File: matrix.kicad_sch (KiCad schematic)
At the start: 94 parts, among them SW10 K08, SW11 K09, SW12 K0A, SW13 K0B, SW14 K0C, SW15 K10, SW16 K11, SW17 K12, SW18 K13, SW19 K14, SW2 K00, SW20 K15, SW21 K16, SW22 K17, SW23 K18, SW24 K19, SW25 K1A, SW26 K1B, SW27 K20, SW28 K21, SW29 K22, SW3 K01, SW30 K23, SW31 K24, SW32 K25, SW33 K26, SW34 K27, SW35 K28, SW36 K29, SW37 K2A, SW38 K2B, SW39 K30, SW4 K02, SW40 K31, SW41 K32, SW42 K33, SW43 K34, SW44 K36, SW45 K38, SW46 K39, SW47 K3A, SW48 K3B, SW5 K03, SW6 K04, SW7 K05, SW8 K06, SW9 K07

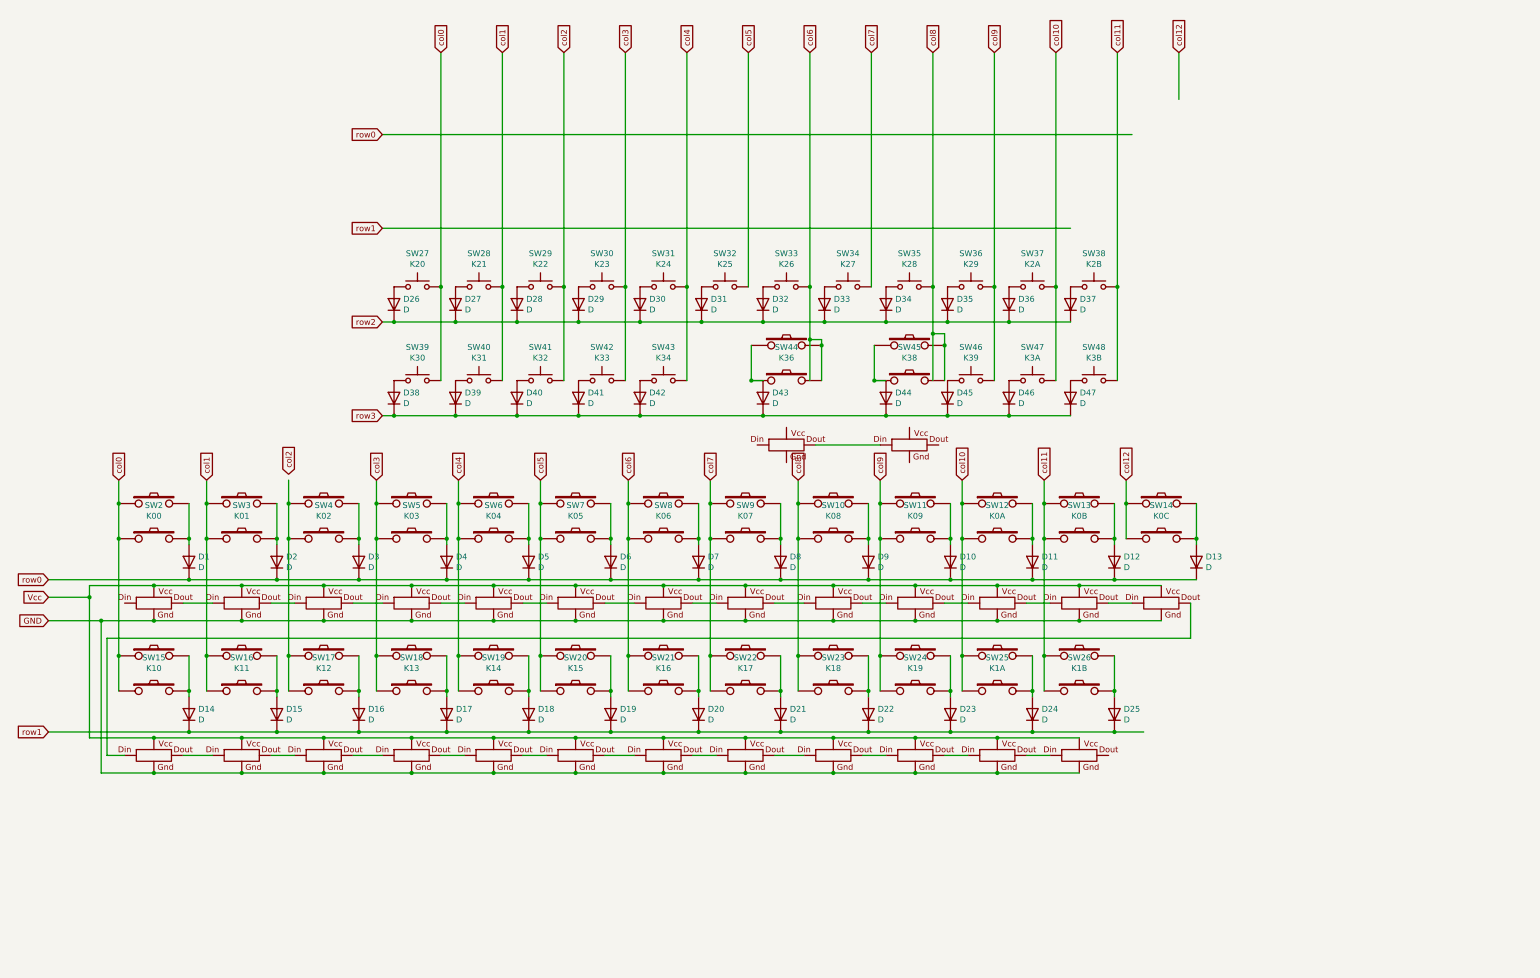
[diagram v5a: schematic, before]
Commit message: routing lol
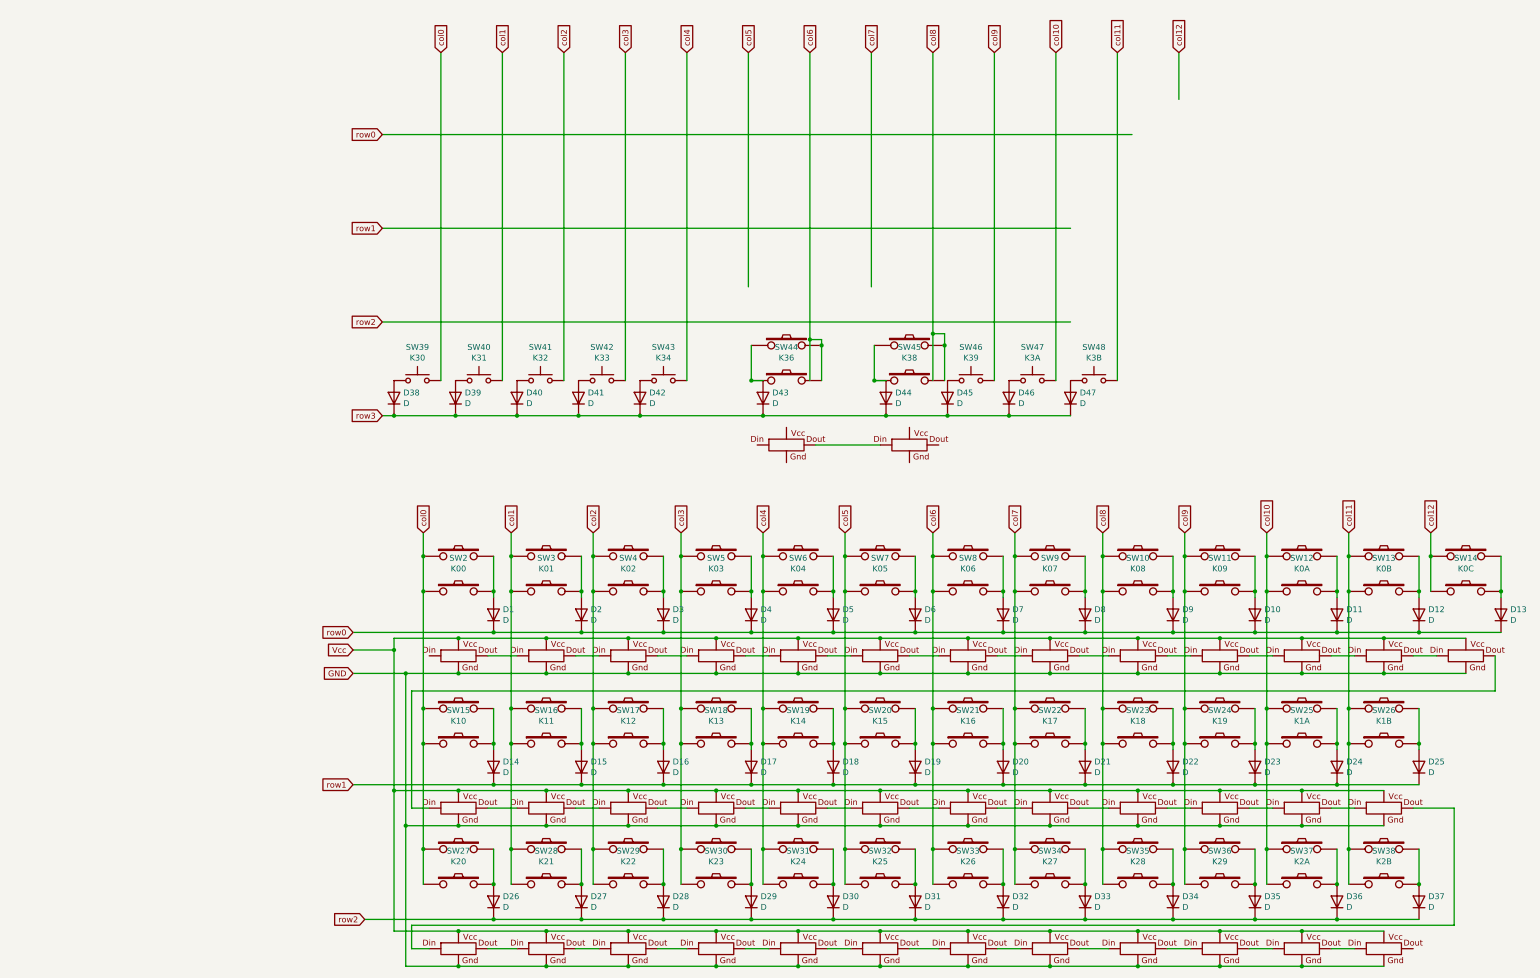
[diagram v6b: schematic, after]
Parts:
- SW27, SW28, SW29, SW30, SW31, SW32, SW33, SW34, SW35, SW36, SW37, SW38: symbol Switch:SW_Push -> switches:SWITCH_PUSH_MXCHOC
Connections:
- net GND: now also SW27.12 (VSS), SW28.12 (VSS), SW29.12 (VSS), SW30.12 (VSS), SW31.12 (VSS), SW32.12 (VSS), SW33.12 (VSS), SW34.12 (VSS), SW35.12 (VSS), SW36.12 (VSS), SW37.12 (VSS), SW38.12 (VSS)
- net Vcc: now also SW27.10 (Vdd), SW28.10 (Vdd), SW29.10 (Vdd), SW30.10 (Vdd), SW31.10 (Vdd), SW32.10 (Vdd), SW33.10 (Vdd), SW34.10 (Vdd), SW35.10 (Vdd), SW36.10 (Vdd), SW37.10 (Vdd), SW38.10 (Vdd)
- net col0: now also SW27.1, SW27.3; no longer SW27.2
- net col1: now also SW28.1, SW28.3; no longer SW28.2
- net col10: now also SW37.1, SW37.3; no longer SW37.2
- net col11: now also SW38.1, SW38.3; no longer SW38.2
- net col2: now also SW17.1, SW17.3, SW29.1, SW29.3, SW4.1, SW4.3; no longer SW29.2
- net col3: now also SW30.1, SW30.3; no longer SW30.2
- net col4: now also SW31.1, SW31.3; no longer SW31.2
- net col5: now also SW32.1, SW32.3; no longer SW32.2
- net col6: now also SW33.1, SW33.3; no longer SW33.2
- net col7: now also SW34.1, SW34.3; no longer SW34.2
- net col8: now also SW35.1, SW35.3; no longer SW35.2
- net col9: now also SW36.1, SW36.3; no longer SW36.2
- net at SW26.9 (Dout): now also SW27.11 (Din)
- net at D28.2 (A): now also SW29.2, SW29.4; no longer SW29.1
- net at D29.2 (A): now also SW30.2, SW30.4; no longer SW30.1
- net at D26.2 (A): now also SW27.2, SW27.4; no longer SW27.1
- net at D27.2 (A): now also SW28.2, SW28.4; no longer SW28.1
- net at D32.2 (A): now also SW33.2, SW33.4; no longer SW33.1
- net at D33.2 (A): now also SW34.2, SW34.4; no longer SW34.1
- net at D37.2 (A): now also SW38.2, SW38.4; no longer SW38.1
- net at D31.2 (A): now also SW32.2, SW32.4; no longer SW32.1
- net at D35.2 (A): now also SW36.2, SW36.4; no longer SW36.1
- net at D34.2 (A): now also SW35.2, SW35.4; no longer SW35.1
- net at D30.2 (A): now also SW31.2, SW31.4; no longer SW31.1
- net at D36.2 (A): now also SW37.2, SW37.4; no longer SW37.1
- new net: SW28.9 (Dout), SW29.11 (Din)
- new net: SW29.9 (Dout), SW30.11 (Din)
- new net: SW30.9 (Dout), SW31.11 (Din)
- new net: SW27.9 (Dout), SW28.11 (Din)
- new net: SW32.9 (Dout), SW33.11 (Din)
- new net: SW33.9 (Dout), SW34.11 (Din)
- new net: SW34.9 (Dout), SW35.11 (Din)
- new net: SW31.9 (Dout), SW32.11 (Din)
- new net: SW35.9 (Dout), SW36.11 (Din)
- new net: SW37.9 (Dout), SW38.11 (Din)
- new net: SW36.9 (Dout), SW37.11 (Din)
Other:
- moved on the sheet: D1, D10, D11, D12, D13, D14, D15, D16, D17, D18, D19, D2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
